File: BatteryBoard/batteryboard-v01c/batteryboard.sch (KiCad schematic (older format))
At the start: 29 parts, among them J1 KEYSTONE-1042, J2 KEYSTONE-1042, J3 KEYSTONE-1042, J4 KEYSTONE-1042, J5 KEYSTONE-1042, J6 KEYSTONE-1042, J7 5023520400, J8 Screw_Terminal_01x02, Q1 IRF7458, Q2 IRF7458, Q3 MMBT2222AT, U1 R5460N233AF

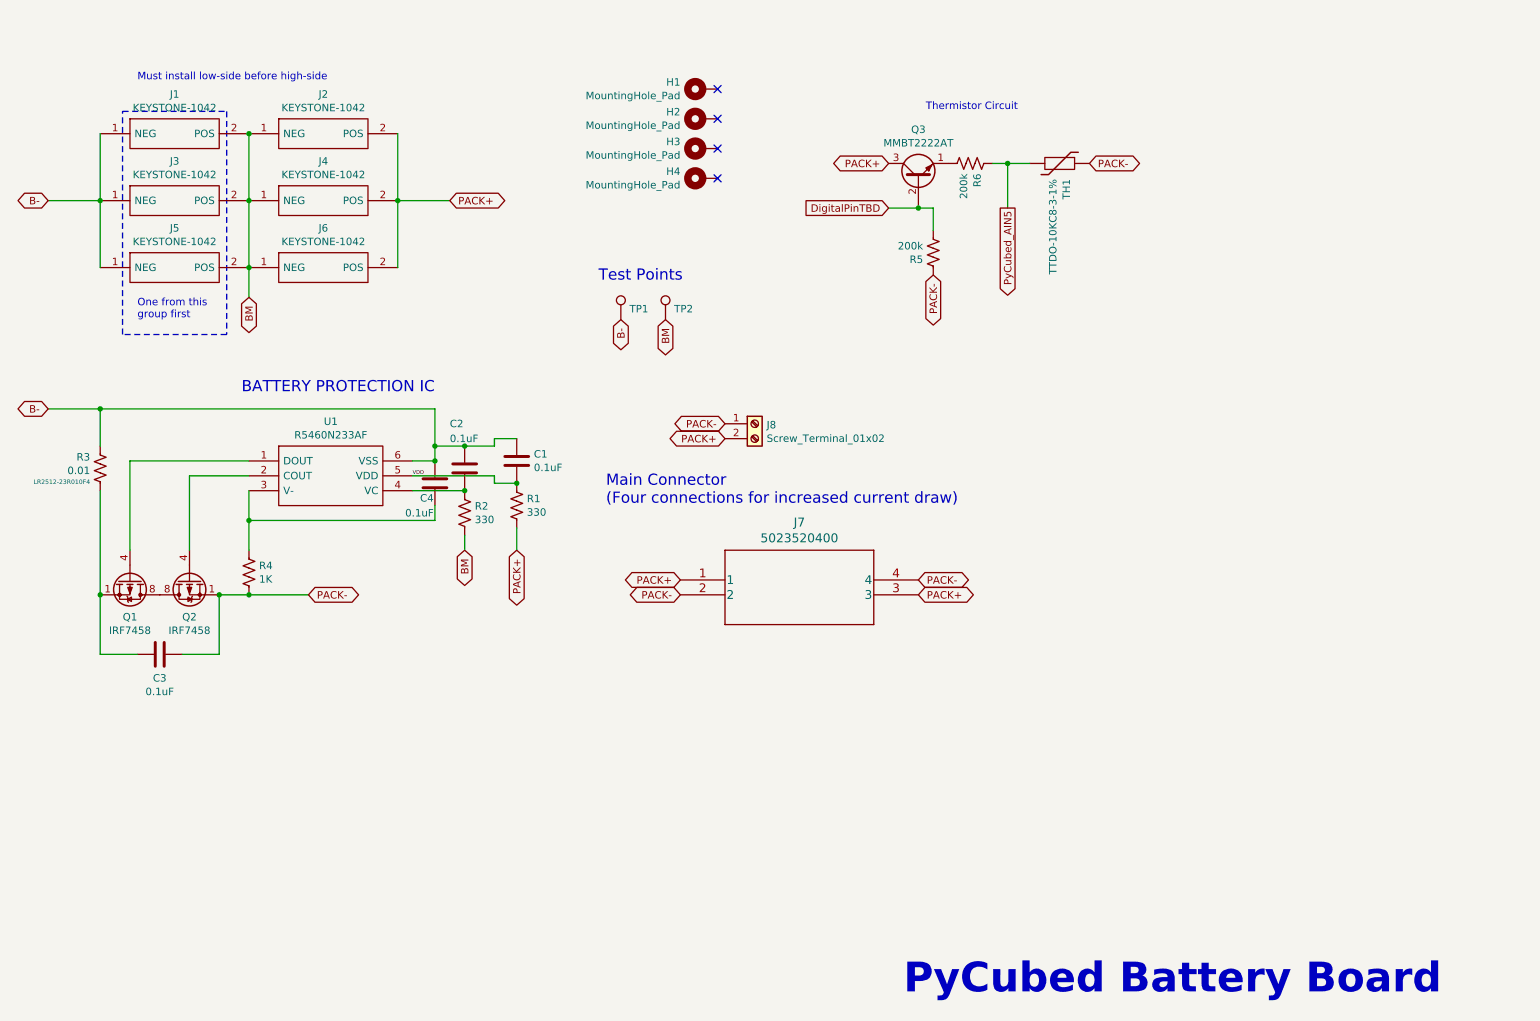
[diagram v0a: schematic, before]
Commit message: Added Sapling Files
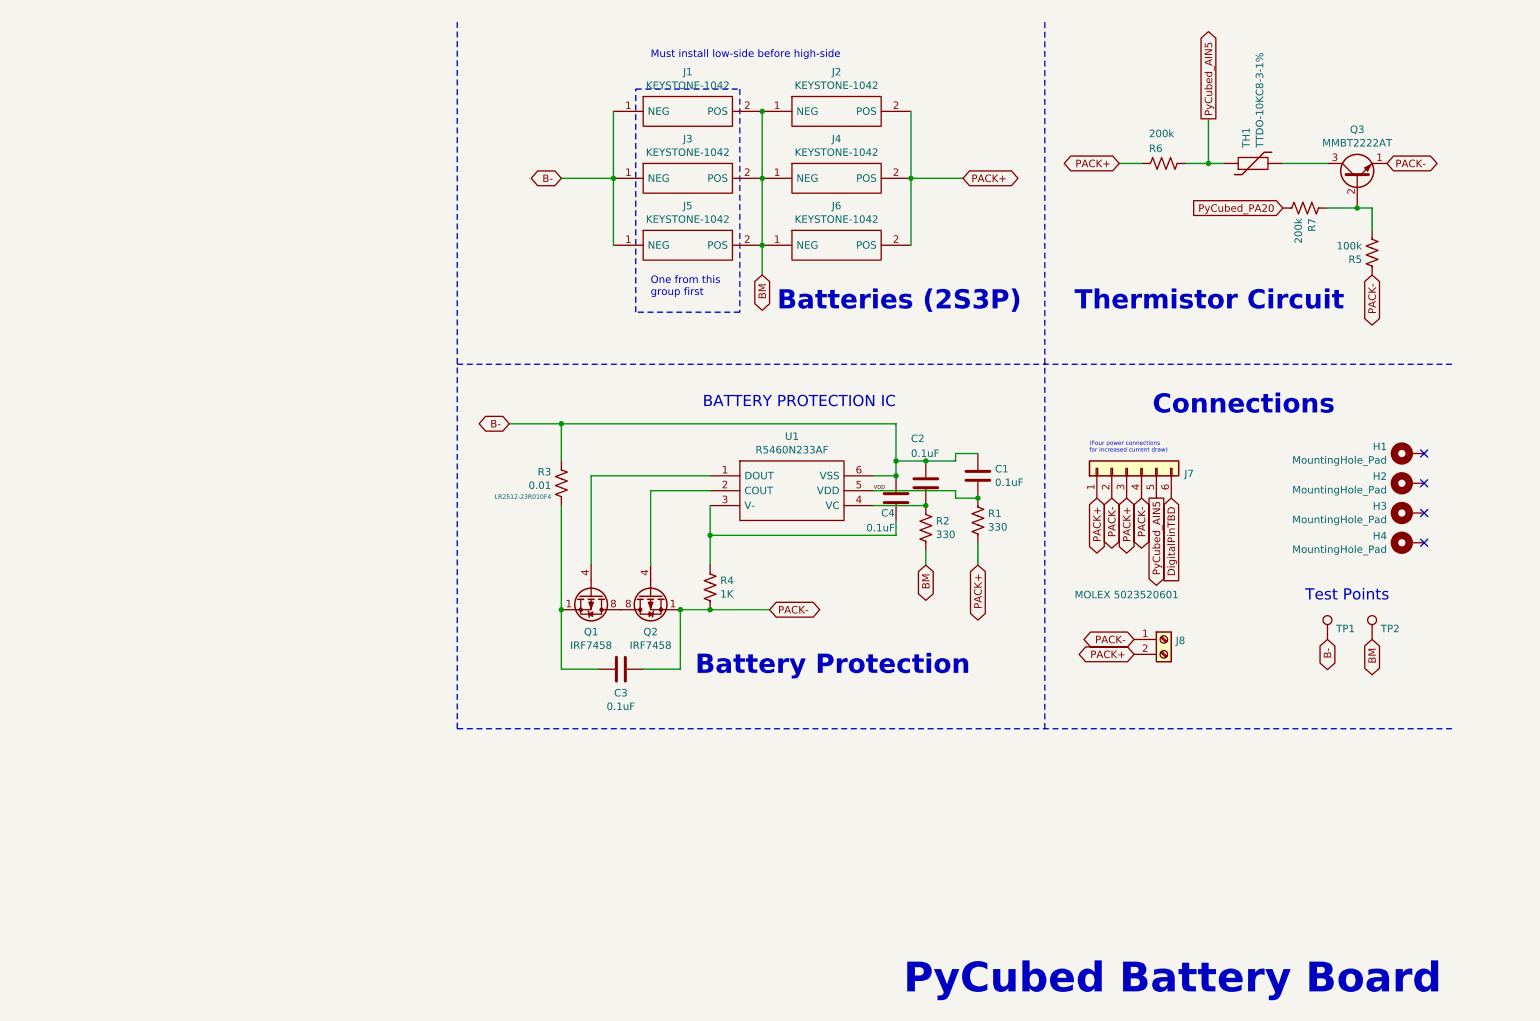
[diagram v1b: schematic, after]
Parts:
- removed J7: 5023520400, batteryboard:duraclik_4pos, symbol batteryboard-rescue:5023520400
- added J7: MOLEX 5023520601, batteryboard:5023520600, symbol Connector_Generic:Conn_01x06
- added R7: 200k, Resistor_SMD:R_0603_1608Metric, symbol Device:R_US
- Q3: footprint Package_TO_SOT_THT:TO-39-3 -> Package_TO_SOT_SMD:SOT-523
- R5: value 200k -> 100k
- R6: footprint Resistor_SMD:R_0603_1608Metric -> Resistor_SMD:R_1206_3216Metric
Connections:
- net DigitalPinTBD: now also J7.6 (Pin_6); no longer Q3.2 (B), R5.1
- net PACK+: now also R6.1, J7.1 (Pin_1), J7.3 (Pin_3); no longer Q3.3 (C)
- net PACK-: now also Q3.1 (E), J7.2 (Pin_2), J7.4 (Pin_4); no longer TH1.1
- net PyCubed_AIN5: now also TH1.1, J7.5 (Pin_5); no longer TH1.2
- new net: Q3.2 (B), R5.1, R7.2
- new net: Q3.3 (C), TH1.2
- new net PyCubed_PA20: R7.1
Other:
- note added: "(Four power connections \nfor increased current draw)"
- note added: "Batteries (2S3P)"
- note added: "Battery Protection"
- note added: "Connections"
- note removed: "Main Connector\n(Four connections for increased current draw)"
- moved on the sheet: C1, C2, C3, C4, H1, H2, H3, H4, J1, J2, J3, J4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
